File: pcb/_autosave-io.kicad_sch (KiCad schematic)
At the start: 53 parts, among them J4 LASER, J6 TT143AMC12C, Q1 BSS214NW, U1 LSM6DSOXTR, U10 MAX30102, U11 TPS65631W, U12 TXB0102YZP, U14 LIS3MDL, U16 DRV2605LDGS, U7 LPS22DF, U8 TCA9406DC

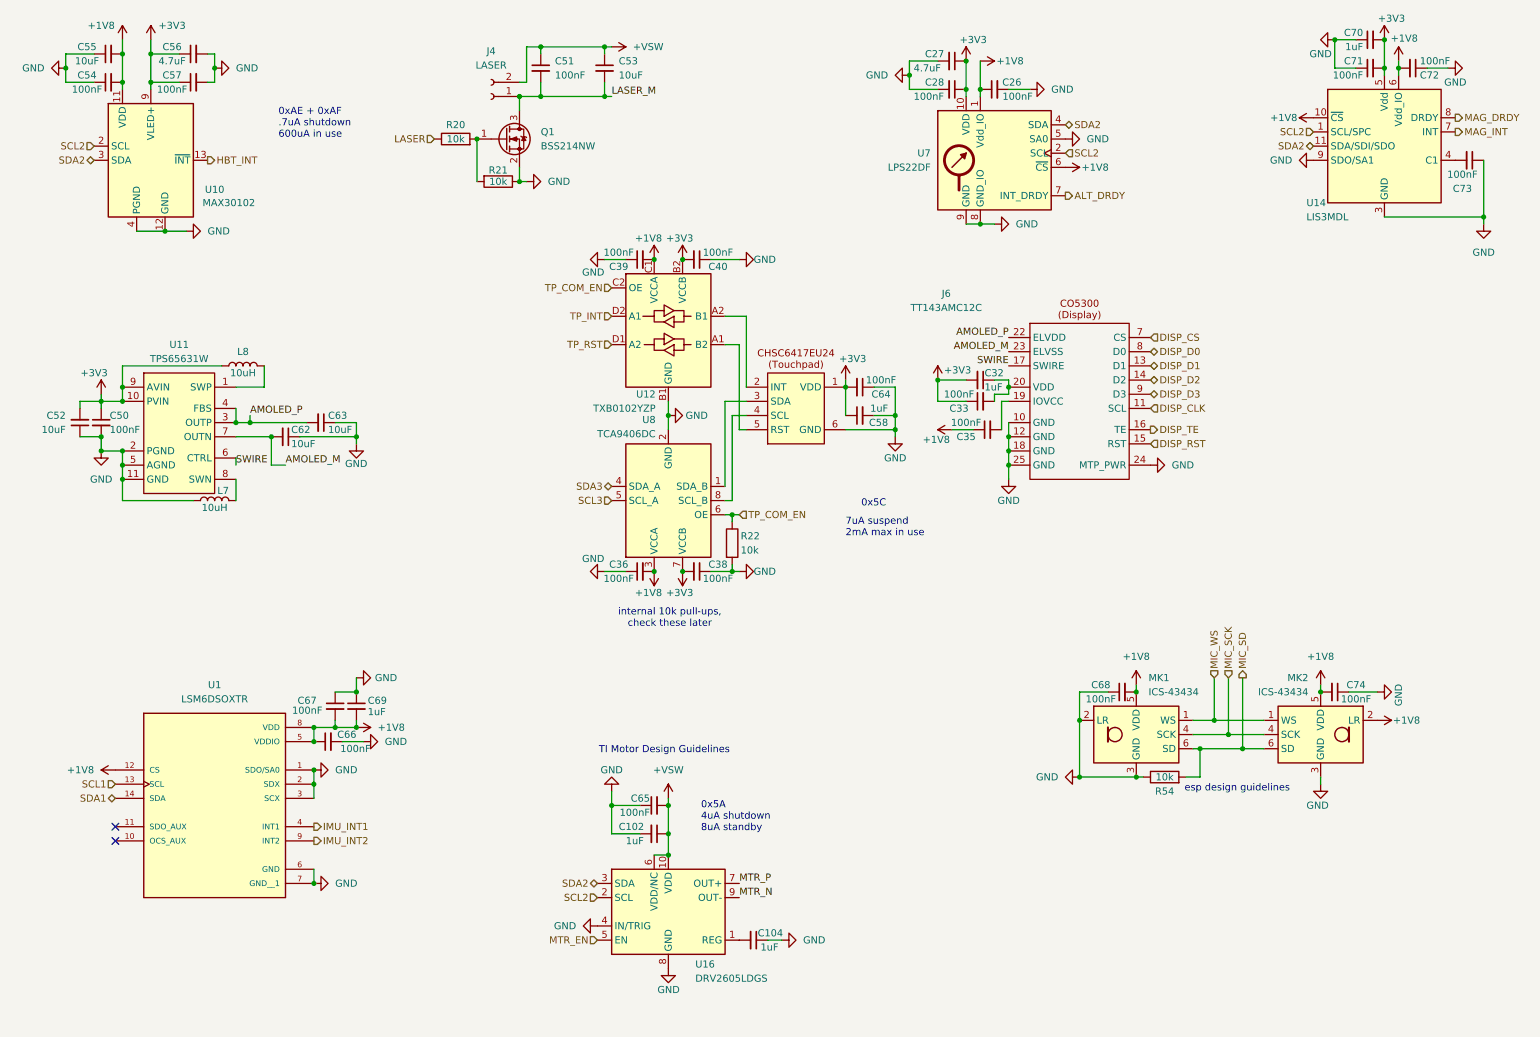
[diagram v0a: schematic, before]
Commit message: returning and reorganizing
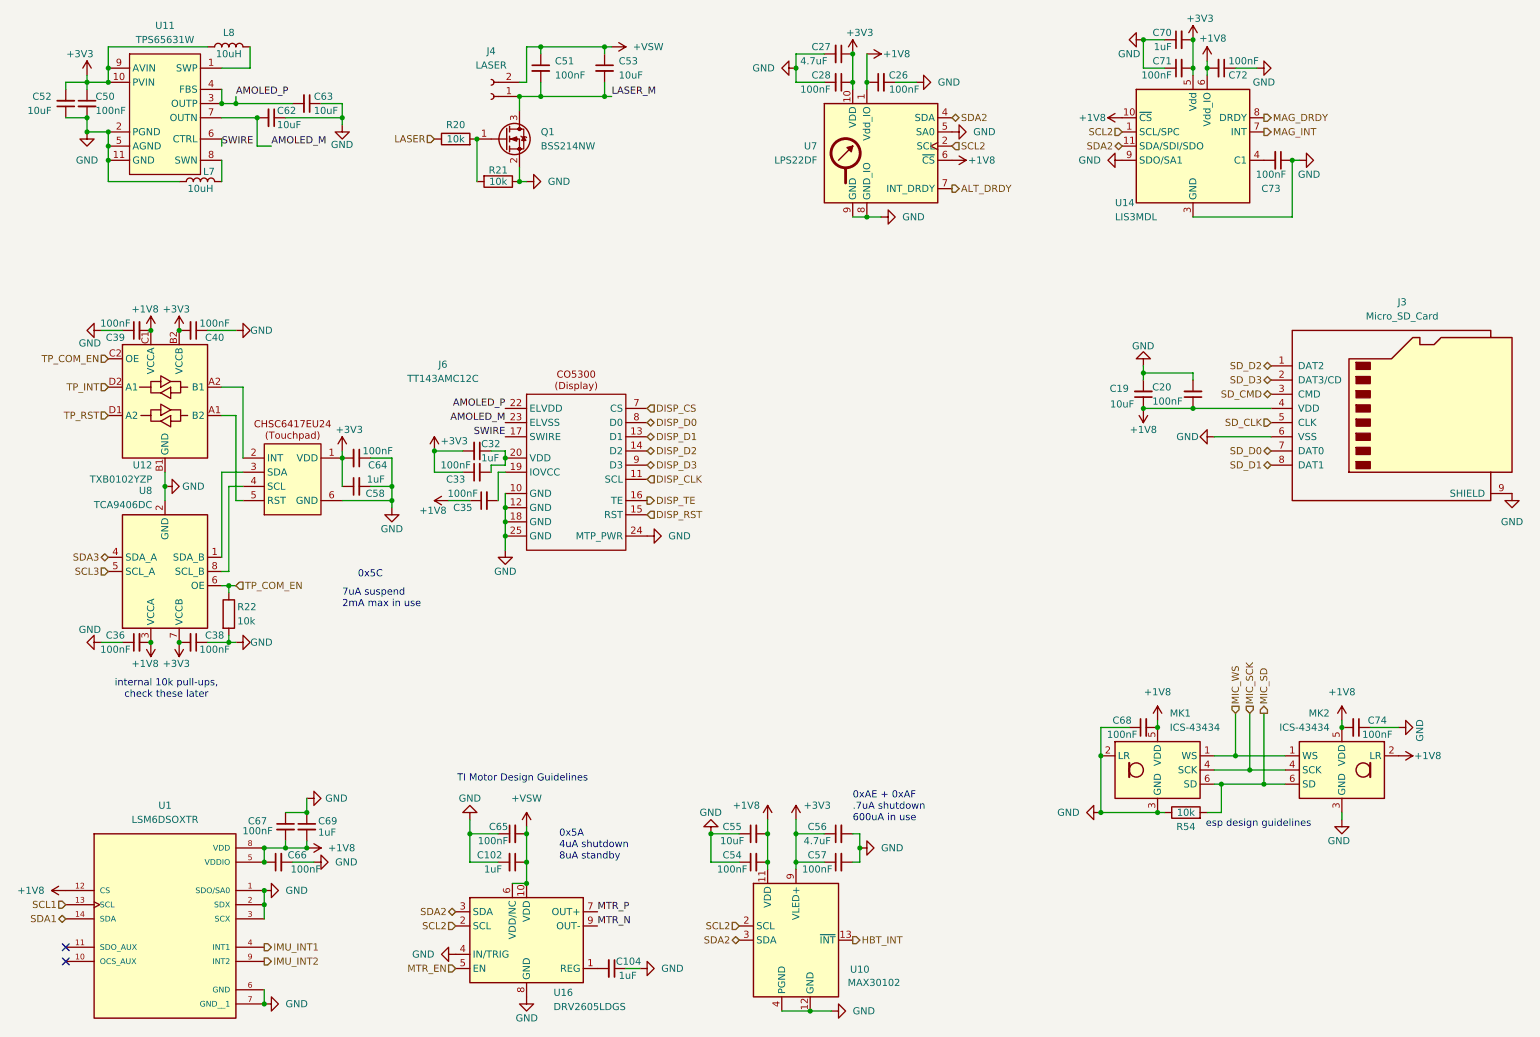
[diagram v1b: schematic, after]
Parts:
- added C19: 10uF, symbol Device:C_Small
- added C20: 100nF, symbol Device:C_Small
- added J3: Micro_SD_Card, Connector_Card:microSD_HC_Molex_104031-0811, symbol Connector:Micro_SD_Card
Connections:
- net +1V8: now also C19.1, C20.1, J3.4 (VDD)
- net GND: now also C19.2, C20.2, J3.6 (VSS), J3.9 (SHIELD)
- new net SD_CLK: J3.5 (CLK)
- new net SD_CMD: J3.3 (CMD)
- new net SD_D0: J3.7 (DAT0)
- new net SD_D1: J3.8 (DAT1)
- new net SD_D2: J3.1 (DAT2)
- new net SD_D3: J3.2 (DAT3/CD)
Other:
- moved on the sheet: C102, C104, C26, C27, C28, C32, C33, C35, C36, C38, C39, C40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
